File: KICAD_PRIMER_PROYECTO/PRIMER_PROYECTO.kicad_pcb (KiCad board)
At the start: 2 copper layers, 16 parts, among them SW1 ON-OFF, SW2 Start, SW3 5 min, SW4 10 min, SW5 15 min, SW6 20 min, U1 NE555P

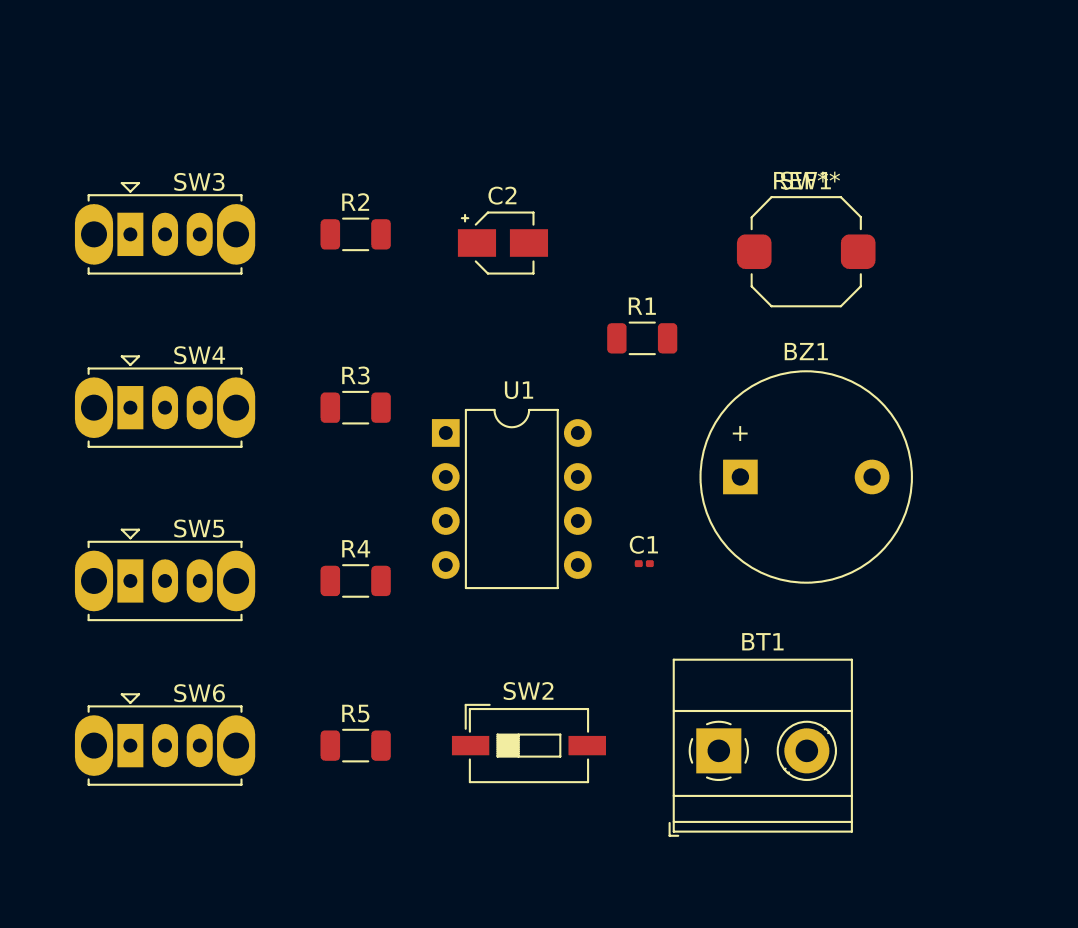
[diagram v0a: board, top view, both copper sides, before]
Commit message: Avance KICAD PCB
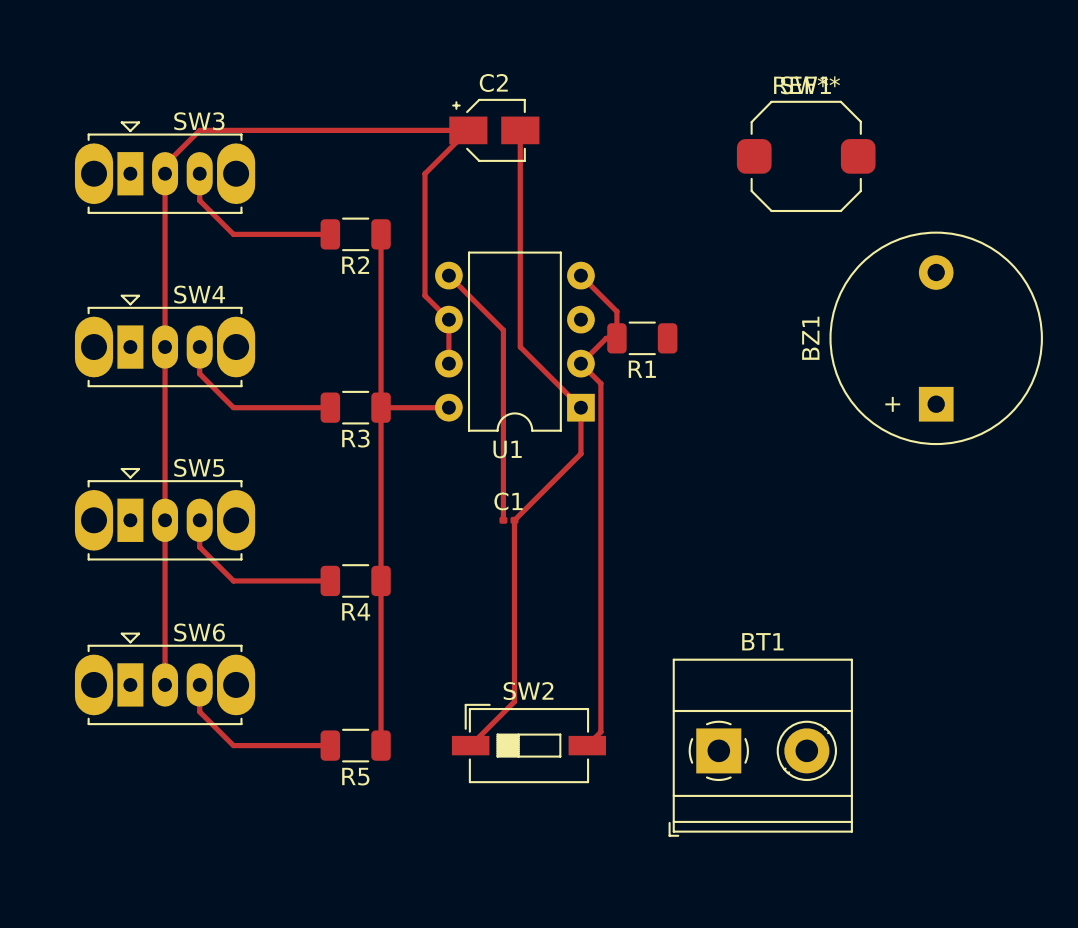
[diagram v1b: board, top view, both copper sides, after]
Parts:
- moved BZ1 12.1 mm to (161.0, 88.8), turned to 90 degrees
- moved C1 8.20 mm to (136.3, 95.5)
- moved U1 7.94 mm to (140.5, 89.0), turned to 180 degrees
- moved C2 6.52 mm to (135.5, 73.0)
- moved SW1 5.50 mm to (153.5, 74.5)
- moved SW3 3.50 mm to (114.5, 75.5)
- moved SW4 3.50 mm to (114.5, 85.5)
- moved SW5 3.50 mm to (114.5, 95.5)
- moved SW6 3.50 mm to (114.5, 105.0)
- turned R1 to 180 degrees
- turned R2 to 180 degrees
- turned R3 to 180 degrees
- turned R4 to 180 degrees
- turned R5 to 180 degrees
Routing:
- net Net-(SW3-B): track 0.00 -> 63.4 mm
- net Net-(BT1--): track 0.00 -> 39.6 mm
- net Net-(BZ1-+): track 0.00 -> 33.4 mm
- net Net-(U1-R): track 0.00 -> 30.0 mm
- net Net-(U1-CV): track 0.00 -> 15.4 mm
- net Net-(SW6-C): track 0.00 -> 9.90 mm
- net Net-(SW5-C): track 0.00 -> 9.90 mm
- net Net-(SW4-C): track 0.00 -> 9.90 mm
- net Net-(SW3-C): track 0.00 -> 9.90 mm

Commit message: Actualizacion KICAD PCB
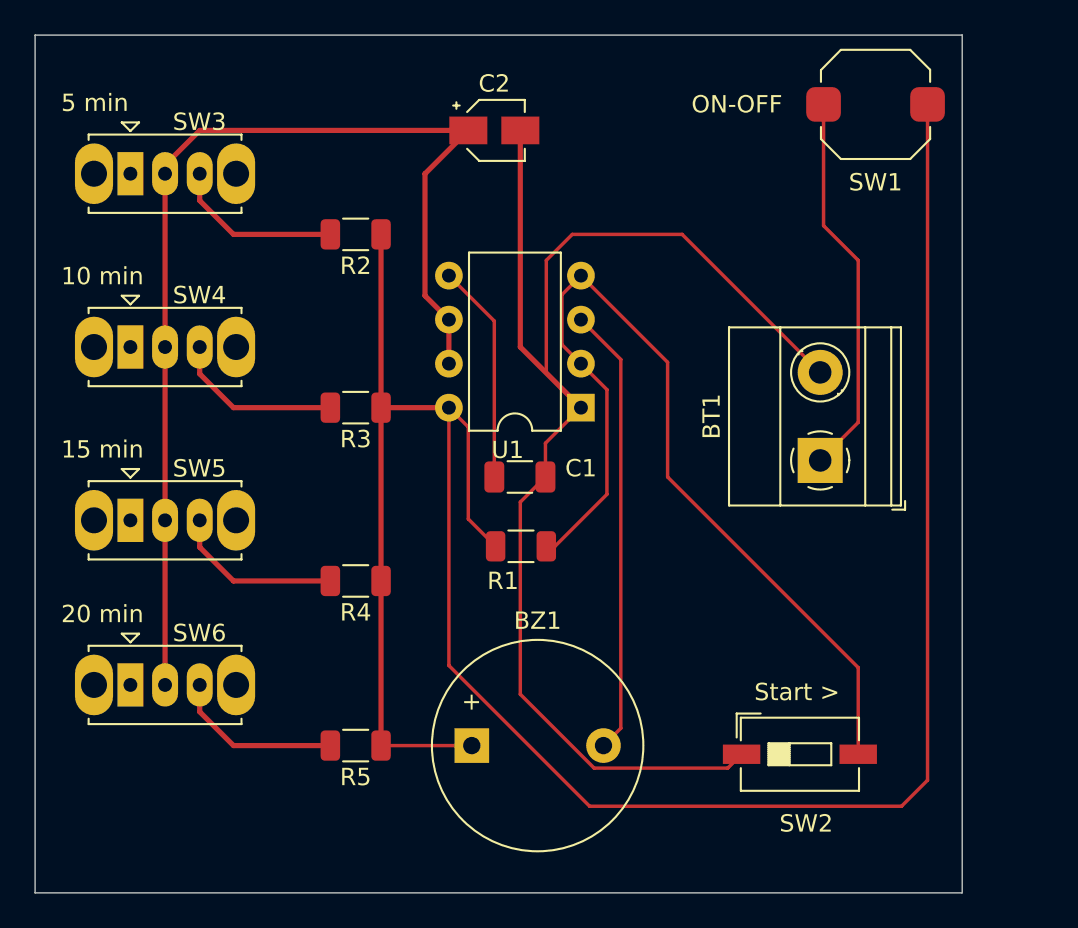
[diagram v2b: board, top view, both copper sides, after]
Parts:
- C1: footprint Capacitor_SMD:C_0201_0603Metric -> Capacitor_SMD:C_1206_3216Metric
- moved BZ1 33.3 mm to (134.2, 108.5), turned to 0 degrees
- moved BT1 17.8 mm to (154.3, 92.0), turned to 90 degrees
- moved SW2 15.6 mm to (153.1, 109.0)
- moved R1 13.9 mm to (137.0, 97.0), turned to 0 degrees
- moved SW1 5.00 mm to (157.5, 71.5)
- moved C1 2.58 mm to (137.0, 93.0)
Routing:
- net Net-(BZ1-+): track 33.4 -> 133.3 mm
- net Net-(BT1--): track 39.6 -> 79.4 mm
- net Net-(BZ1--): track 0.00 -> 25.9 mm
- net Net-(U1-R): track 30.0 -> 53.1 mm
- net Net-(BT1-+): track 0.00 -> 22.3 mm
- net Net-(U1-CV): track 15.4 -> 12.7 mm
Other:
- board outline added: 53.5 x 49.5 mm
- board text added: "10 min"
- board text added: "15 min"
- board text added: "20 min"
- board text added: "5 min"
- board text added: "Start >"
